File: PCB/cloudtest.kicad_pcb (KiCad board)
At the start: 2 copper layers, 35.5 x 36.5 mm, 10 parts, among them J1 PulseIn, J2 Display, U1 ESP32-C3_SUPERMINI_TH, U2 MIC5219-5.0YM5, U3 MIC5219-3.3YM5

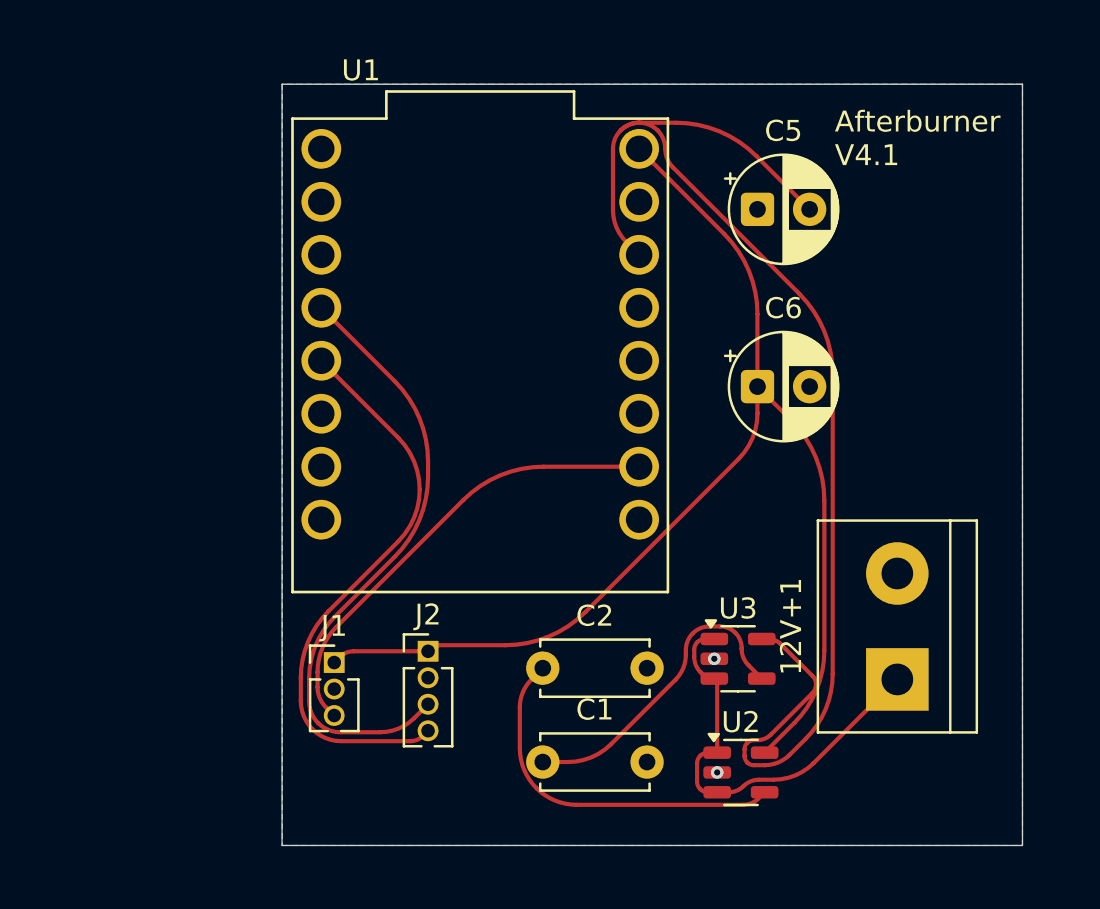
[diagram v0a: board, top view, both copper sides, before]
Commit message: Fixed PCB (hopefully)
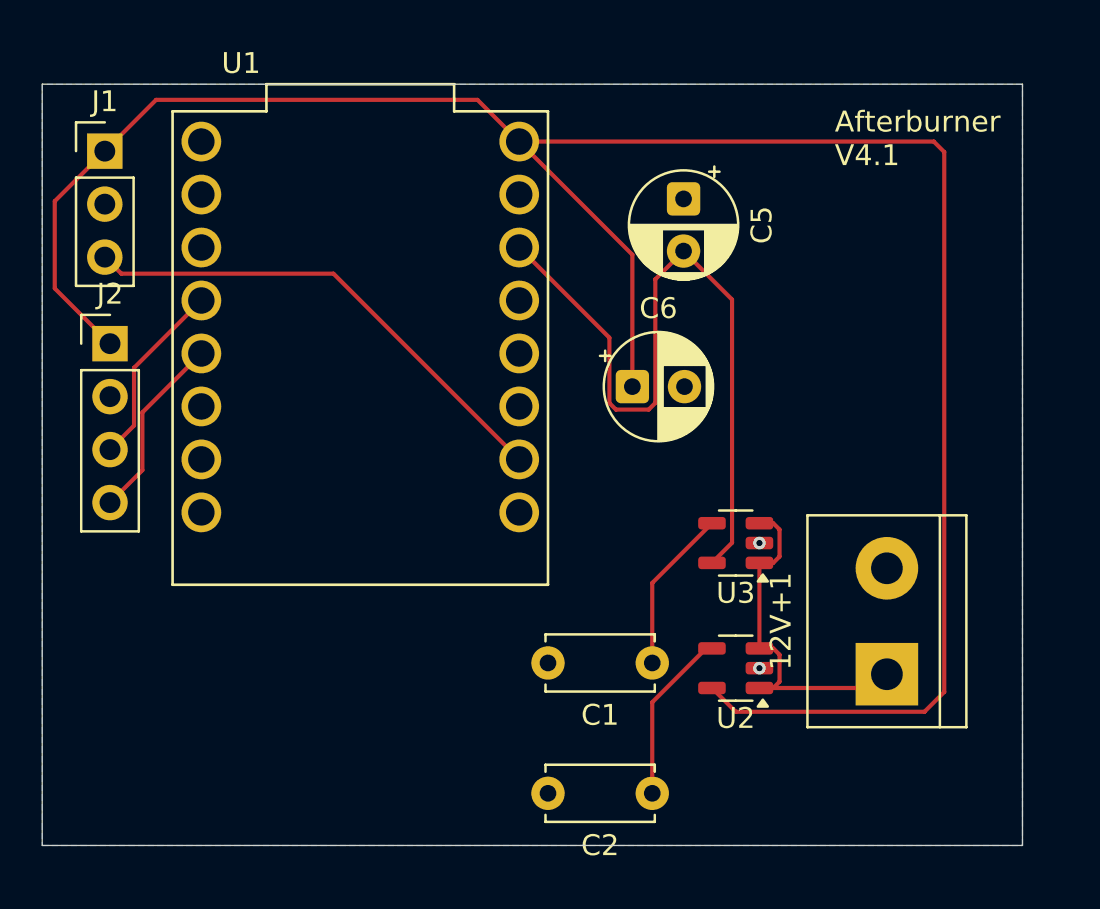
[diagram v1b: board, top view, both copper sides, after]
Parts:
- J1: footprint Connector_PinHeader_1.27mm:PinHeader_1x03_P1.27mm_Vertical -> Connector_PinHeader_2.54mm:PinHeader_1x03_P2.54mm_Vertical
- J2: footprint Connector_PinHeader_1.27mm:PinHeader_1x04_P1.27mm_Vertical -> Connector_PinHeader_2.54mm:PinHeader_1x04_P2.54mm_Vertical
- moved J1 26.9 mm to (23.5, 65.2)
- moved J2 21.2 mm to (23.8, 74.4)
- moved C2 7.97 mm to (49.8, 96.0), turned to 180 degrees
- moved C1 7.08 mm to (49.8, 89.8), turned to 180 degrees
- moved C6 6.00 mm to (48.8, 76.5)
- moved U1 5.76 mm to (35.8, 74.7)
- moved U3 5.55 mm to (53.8, 84.0), turned to 180 degrees
- moved U2 5.01 mm to (53.8, 90.0), turned to 180 degrees
- moved C5 3.58 mm to (51.2, 67.5), turned to -90 degrees
- moved 12V+1 0.56 mm to (61.0, 90.3)
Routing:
- net VCC: track 59.8 -> 105.7 mm
- net +3.3V: track 64.0 -> 35.9 mm
- net /i2c esp sda: track 29.6 -> 8.96 mm
- net /i2c esp sdc: track 27.4 -> 8.96 mm
- net Net-(U2-BP): track 17.7 -> 8.30 mm
- net Net-(U3-BP): track 15.1 -> 7.89 mm
- net +12V: track 20.6 -> 17.4 mm
- net Net-(J1-Pin_3): track 22.2 -> 23.9 mm
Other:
- board size 35.5 x 36.5 mm -> 47 x 36.5 mm
